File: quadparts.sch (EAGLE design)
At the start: 69 parts, among them J1 AVR_SPI_PRG_6NS, U1 ATMEGA128RFA1, Y1 16MHz

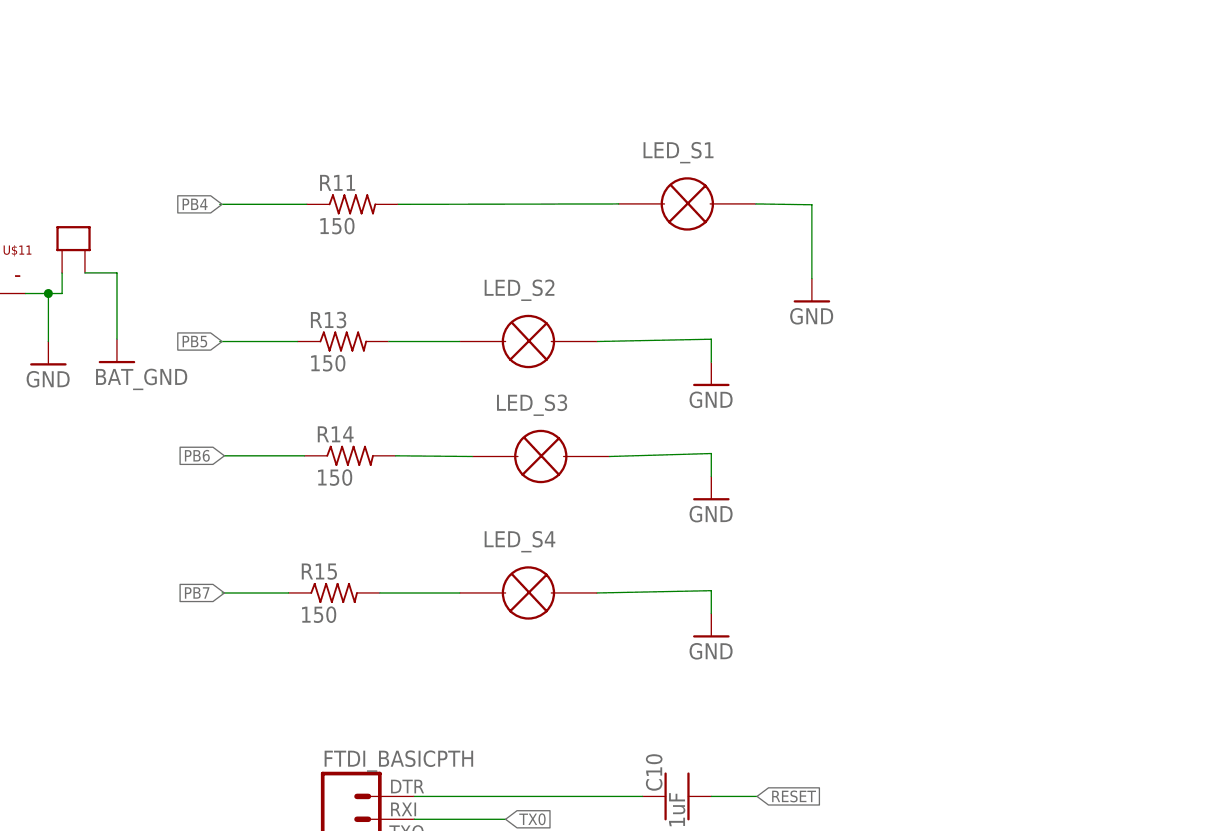
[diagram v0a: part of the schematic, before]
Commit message: Life is so hard
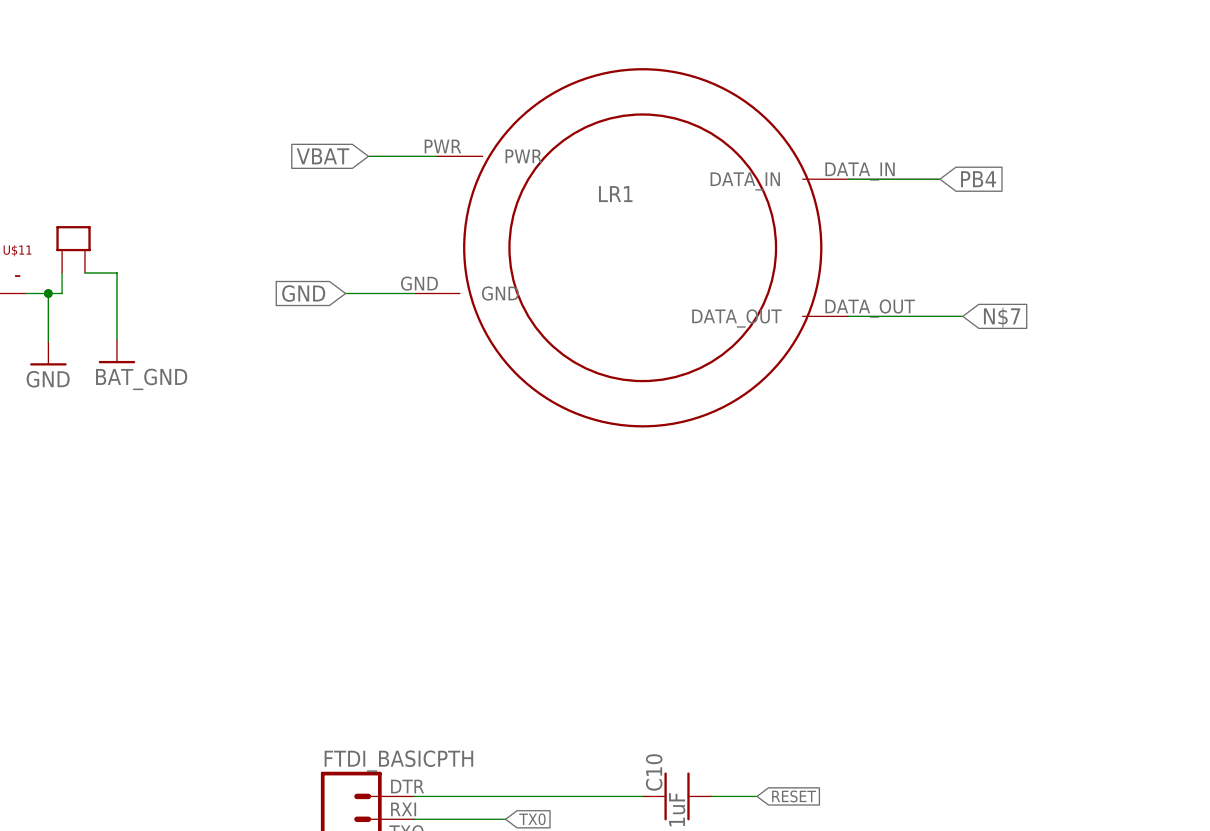
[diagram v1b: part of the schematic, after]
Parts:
- removed LED_S1, LED_S2, LED_S3, LED_S4: (no value), LEDs:LED
- removed R11, R13, R14, R15: 150, quadparts_prebuilt:RESISTOR_SMD-2012-0805-100
- added LR1: LED_RING, LEDs:LED_RING
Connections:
- removed net N$5: LED_S1.P$1, R11.2
- removed net N$6: LED_S2.P$1, R13.2
- removed net N$9: LED_S4.P$1, R15.2
- net GND: now also LR1.GND; no longer LED_S1.P$2, LED_S2.P$2, LED_S3.P$2, LED_S4.P$2
- net N$7: now also LR1.DATA_OUT; no longer LED_S3.P$1, R14.2
- net PB4: now also LR1.DATA_IN; no longer R11.1
- net PB5: no longer R13.1
- net PB6: no longer R14.1
- net PB7: no longer R15.1
- net VBAT: now also LR1.PWR
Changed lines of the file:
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@@
 <setting verticaltext="up"/>
 </settings>
-<grid distance="0.001" unitdist="inch" unit="inch" style="lines" multiple="1" display="no" altdistance="0.01" altunitdist="inch" altunit="inch"/>
+<grid distance="0.1" unitdist="inch" unit="inch" style="lines" multiple="1" display="no" altdistance="0.01" altunitdist="inch" altunit="inch"/>
 <layers>
 <layer number="1" name="Top" color="4" fill="1" visible="no" active="no"/>
@@
 <part name="GND37" library="quadparts_prebuilt" deviceset="GND" device=""/>
 <part name="GND38" library="quadparts_prebuilt" deviceset="BAT_GND" device=""/>
-<part name="GND39" library="quadparts_prebuilt" deviceset="GND" device=""/>
-<part name="GND40" library="quadparts_prebuilt" deviceset="GND" device=""/>
-<part name="GND41" library="quadparts_prebuilt" deviceset="GND" device=""/>
-<part name="GND42" library="quadparts_prebuilt" deviceset="GND" device=""/>
 <part name="C5" library="quadparts_prebuilt" deviceset="CAPACITOR-NP_" device="SMD-2012-0805_CERAMIC-1UF" value="1uF"/>
 <part name="C6" library="quadparts_prebuilt" deviceset="CAPACITOR-NP_" device="SMD-2012-0805_CERAMIC-1UF" value="1uF"/>
@@
 <part name="C28" library="quadparts_prebuilt" deviceset="CAPACITOR-NP_" device="SMD-2012-0805_CERAMIC-1UF" value="1uF"/>
 <part name="C29" library="quadparts_prebuilt" deviceset="CAPACITOR-NP_" device="SMD-2012-0805_CERAMIC-1UF" value="1uF"/>
-<part name="LED_S1" library="LEDs" deviceset="LED" device=""/>
-<part name="LED_S2" library="LEDs" deviceset="LED" device=""/>
-<part name="LED_S3" library="LEDs" deviceset="LED" device=""/>
-<part name="LED_S4" library="LEDs" deviceset="LED" device=""/>
 <part name="J2" library="quadparts_Jason" deviceset="MALE_HEADER_2POS" device="-2X1-0.1IN"/>
 <part name="D1" library="quadparts_prebuilt" deviceset="DIODE-SCHOTTKY_" device="SMD-SOD123-360MV" value="360mV"/>
@@
 <part name="GND24" library="quadparts_prebuilt" deviceset="BAT_GND" device=""/>
 <part name="GND26" library="quadparts_prebuilt" deviceset="BAT_GND" device=""/>
-<part name="R11" library="quadparts_prebuilt" deviceset="RESISTOR_" device="SMD-2012-0805-100" value="150"/>
-<part name="R13" library="quadparts_prebuilt" deviceset="RESISTOR_" device="SMD-2012-0805-100" value="150"/>
-<part name="R14" library="quadparts_prebuilt" deviceset="RESISTOR_" device="SMD-2012-0805-100" value="150"/>
-<part name="R15" library="quadparts_prebuilt" deviceset="RESISTOR_" device="SMD-2012-0805-100" value="150"/>
 <part name="R2" library="quadparts_prebuilt" deviceset="RESISTOR_" device="SMD-2012-0805-10K" value="10K"/>
 <part name="R3" library="quadparts_prebuilt" deviceset="RESISTOR_" device="SMD-2012-0805-10K" value="10K"/>
@@
 <part name="C3" library="quadparts_prebuilt" deviceset="CAPACITOR-NP_" device="SMD-2012-0805_CERAMIC-0.1UF" value="0.1uF"/>
 <part name="C4" library="quadparts_prebuilt" deviceset="CAPACITOR-NP_" device="SMD-2012-0805_CERAMIC-0.1UF" value="0.1uF"/>
+<part name="LR1" library="LEDs" deviceset="LED_RING" device=""/>
 </parts>
 <sheets>
@@
 <instance part="GND37" gate="1" x="-15.24" y="200.66"/>
 <instance part="GND38" gate="1" x="88.9" y="200.66"/>
-<instance part="GND39" gate="1" x="166.116" y="207.404"/>
-<instance part="GND40" gate="1" x="154.94" y="198.12"/>
-<instance part="GND41" gate="1" x="154.94" y="185.42"/>
-<instance part="GND42" gate="1" x="154.94" y="170.18"/>
 <instance part="C5" gate="G$1" x="38.1" y="114.3" rot="R180"/>
 <instance part="C6" gate="G$1" x="48.26" y="114.3" rot="R180"/>
@@
 <instance part="C28" gate="G$1" x="96.52" y="33.02"/>
 <instance part="C29" gate="G$1" x="104.14" y="33.02"/>
-<instance part="LED_S1" gate="G$1" x="152.274" y="218.232"/>
-<instance part="LED_S2" gate="G$1" x="134.62" y="202.946"/>
-<instance part="LED_S3" gate="G$1" x="135.9916" y="190.1698"/>
-<instance part="LED_S4" gate="G$1" x="134.62" y="175.006"/>
 <instance part="J2" gate="G$1" x="43.18" y="205.74" rot="R270"/>
 <instance part="D1" gate="G$1" x="224.79" y="17.78" rot="R90"/>
@@
 <instance part="GND24" gate="1" x="261.62" y="-41.148"/>
 <instance part="GND26" gate="1" x="337.82" y="-41.402"/>
-<instance part="R11" gate="G$1" x="115.062" y="218.186"/>
-<instance part="R13" gate="G$1" x="114.046" y="202.946"/>
-<instance part="R14" gate="G$1" x="114.808" y="190.246"/>
-<instance part="R15" gate="G$1" x="113.03" y="175.006"/>
 <instance part="R2" gate="G$1" x="218.487" y="121.36" rot="R270"/>
 <instance part="R3" gate="G$1" x="212.3402" y="121.106" rot="R270"/>
@@
 <instance part="C3" gate="G$1" x="264.16" y="-22.352"/>
 <instance part="C4" gate="G$1" x="340.36" y="-19.812"/>
+<instance part="LR1" gate="G$1" x="147.32" y="213.36"/>
 </instances>
 <busses>
@@
 </segment>
 <segment>
-<pinref part="R11" gate="G$1" pin="1"/>
-<wire x1="109.982" y1="218.186" x2="100.33" y2="218.186" width="0.1524" layer="91"/>
-<label x="100.584" y="218.186" size="1.27" layer="95" rot="R180" xref="yes"/>
+<pinref part="LR1" gate="G$1" pin="DATA_IN"/>
+<wire x1="170.18" y1="220.98" x2="180.34" y2="220.98" width="0.1524" layer="91"/>
+<label x="180.34" y="220.98" size="1.778" layer="95" xref="yes"/>
 </segment>
 </net>
@@
 </segment>
 <segment>
-<pinref part="R13" gate="G$1" pin="1"/>
-<wire x1="108.966" y1="202.946" x2="100.33" y2="202.946" width="0.1524" layer="91"/>
-<label x="100.584" y="202.946" size="1.27" layer="95" rot="R180" xref="yes"/>
-</segment>
-<segment>
 <wire x1="90.1192" y1="-4.7244" x2="94.234" y2="-4.699" width="0.1524" layer="91"/>
 <pinref part="R12" gate="G$1" pin="1"/>
@@
 <label x="5.08" y="81.28" size="1.27" layer="95" rot="R180" xref="yes"/>
 </segment>
-<segment>
-<pinref part="R14" gate="G$1" pin="1"/>
-<wire x1="109.728" y1="190.246" x2="100.838" y2="190.246" width="0.1524" layer="91"/>
-<label x="100.838" y="190.246" size="1.27" layer="95" rot="R180" xref="yes"/>
-</segment>
 </net>
 <net name="PB7" class="0">
@@
 <wire x1="12.7" y1="78.74" x2="5.08" y2="78.74" width="0.1524" layer="91"/>
 <label x="5.08" y="78.74" size="1.27" layer="95" rot="R180" xref="yes"/>
-</segment>
-<segment>
-<pinref part="R15" gate="G$1" pin="1"/>
-<wire x1="107.95" y1="175.006" x2="100.584" y2="175.006" width="0.1524" layer="91"/>
-<label x="100.838" y="175.006" size="1.27" layer="95" rot="R180" xref="yes"/>
 </segment>
 </net>
@@
 </segment>
 <segment>
-<pinref part="GND41" gate="1" pin="GND"/>
-<wire x1="143.6116" y1="190.1698" x2="154.94" y2="190.5" width="0.1524" layer="91"/>
-<wire x1="154.94" y1="190.5" x2="154.94" y2="187.96" width="0.1524" layer="91"/>
-<pinref part="LED_S3" gate="G$1" pin="P$2"/>
-</segment>
-<segment>
-<pinref part="GND42" gate="1" pin="GND"/>
-<wire x1="142.24" y1="175.006" x2="154.94" y2="175.26" width="0.1524" layer="91"/>
-<wire x1="154.94" y1="175.26" x2="154.94" y2="172.72" width="0.1524" layer="91"/>
-<pinref part="LED_S4" gate="G$1" pin="P$2"/>
-</segment>
-<segment>
 <pinref part="U1" gate="G$1" pin="PG4(TOSC1)"/>
 <wire x1="12.7" y1="17.78" x2="-2.54" y2="17.78" width="0.1524" layer="91"/>
@@
 <wire x1="68.58" y1="17.78" x2="68.58" y2="5.08" width="0.1524" layer="91"/>
 <pinref part="GND8" gate="1" pin="GND"/>
-</segment>
-<segment>
-<pinref part="LED_S2" gate="G$1" pin="P$2"/>
-<pinref part="GND40" gate="1" pin="GND"/>
-<wire x1="142.24" y1="202.946" x2="154.94" y2="203.2" width="0.1524" layer="91"/>
-<wire x1="154.94" y1="203.2" x2="154.94" y2="200.66" width="0.1524" layer="91"/>
-</segment>
-<segment>
-<pinref part="LED_S1" gate="G$1" pin="P$2"/>
-<pinref part="GND39" gate="1" pin="GND"/>
-<wire x1="159.894" y1="218.232" x2="166.116" y2="218.14" width="0.1524" layer="91"/>
-<wire x1="166.116" y1="218.14" x2="166.116" y2="209.944" width="0.1524" layer="91"/>
 </segment>
 <segment>
@@
 <wire x1="168.148" y1="127" x2="174.244" y2="127" width="0.1524" layer="91"/>
 <wire x1="174.244" y1="127" x2="174.244" y2="121.158" width="0.1524" layer="91"/>
+</segment>
+<segment>
+<pinref part="LR1" gate="G$1" pin="GND"/>
+<wire x1="121.92" y1="208.28" x2="114.3" y2="208.28" width="0.1524" layer="91"/>
+<label x="114.3" y="208.28" size="1.778" layer="95" rot="R180" xref="yes"/>
 </segment>
 </net>
@@
 <wire x1="304.8" y1="18.542" x2="304.8" y2="21.59" width="0.1524" layer="91"/>
 <junction x="271.78" y="21.59"/>
+</segment>
+<segment>
+<pinref part="LR1" gate="G$1" pin="PWR"/>
+<wire x1="124.46" y1="223.52" x2="116.84" y2="223.52" width="0.1524" layer="91"/>
+<label x="116.84" y="223.52" size="1.778" layer="95" rot="R180" xref="yes"/>
 </segment>
 </net>
@@
 </segment>
 </net>
-<net name="N$5" class="0">
-<segment>
-<pinref part="R11" gate="G$1" pin="2"/>
-<pinref part="LED_S1" gate="G$1" pin="P$1"/>
-<wire x1="120.142" y1="218.186" x2="144.654" y2="218.232" width="0.1524" layer="91"/>
-</segment>
-</net>
-<net name="N$6" class="0">
-<segment>
-<pinref part="R13" gate="G$1" pin="2"/>
-<pinref part="LED_S2" gate="G$1" pin="P$1"/>
-<wire x1="119.126" y1="202.946" x2="127" y2="202.946" width="0.1524" layer="91"/>
-</segment>
-</net>
-<net name="N$7" class="0">
-<segment>
-<pinref part="R14" gate="G$1" pin="2"/>
-<pinref part="LED_S3" gate="G$1" pin="P$1"/>
-<wire x1="119.888" y1="190.246" x2="128.3716" y2="190.1698" width="0.1524" layer="91"/>
-</segment>
-</net>
-<net name="N$9" class="0">
-<segment>
-<pinref part="R15" gate="G$1" pin="2"/>
-<pinref part="LED_S4" gate="G$1" pin="P$1"/>
-<wire x1="118.11" y1="175.006" x2="127" y2="175.006" width="0.1524" layer="91"/>
-</segment>
-</net>
 <net name="N$2" class="0">
 <segment>
@@
 </segment>
 </net>
+<net name="N$7" class="0">
+<segment>
+<pinref part="LR1" gate="G$1" pin="DATA_OUT"/>
+<wire x1="170.18" y1="205.74" x2="182.88" y2="205.74" width="0.1524" layer="91"/>
+<label x="182.88" y="205.74" size="1.778" layer="95" xref="yes"/>
+</segment>
+</net>
